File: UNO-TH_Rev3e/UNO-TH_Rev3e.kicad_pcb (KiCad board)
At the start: 2 copper layers, 68.6 x 53.3 mm, 120 parts, among them T1 FDN340P, U1 NCP1117ST50T3G, U2 LP2985-33DBVR, U3 ATMEGA16U2-MU(R), U5 LMV358IDGKR, X1 POWERSUPPLY_DC21MMX, X2 USB-B_TH, Y1 16MHz, Y2 CSTCE16M0V53-R0 16MHZ

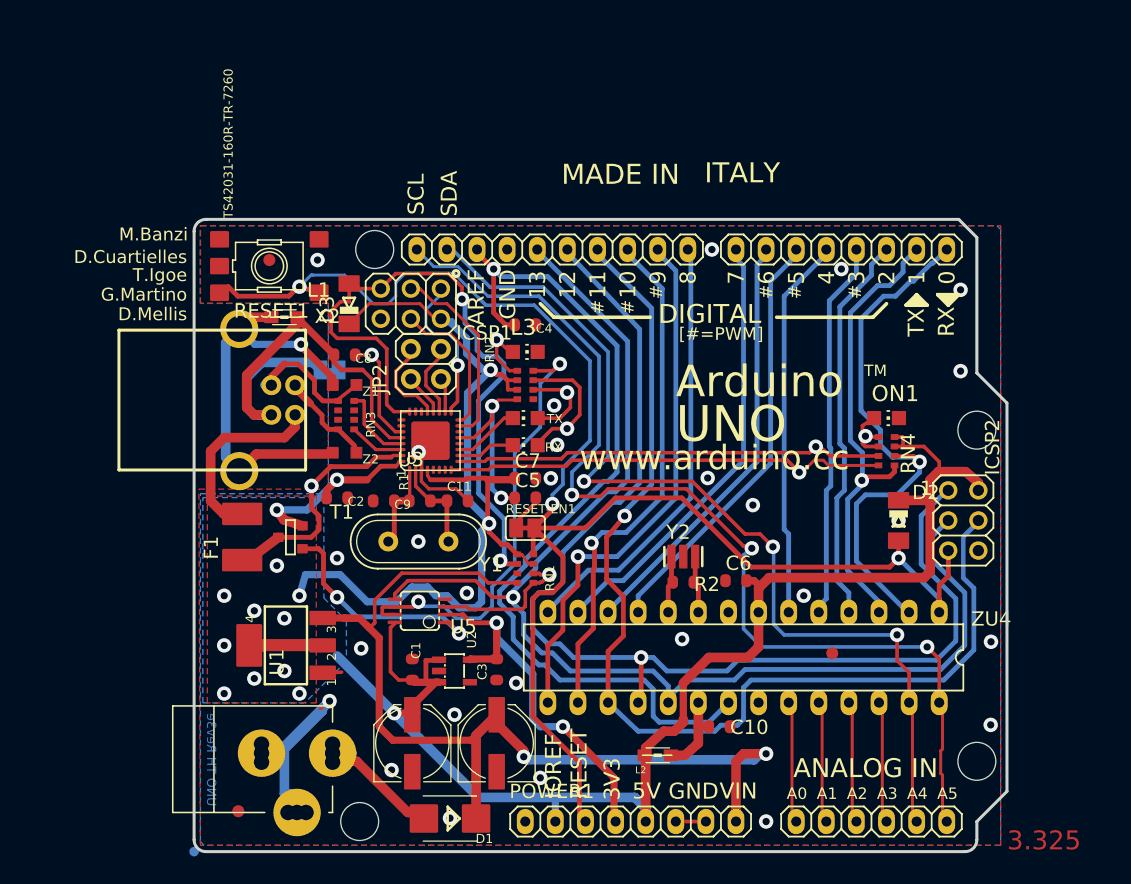
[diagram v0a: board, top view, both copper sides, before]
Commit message: rasp
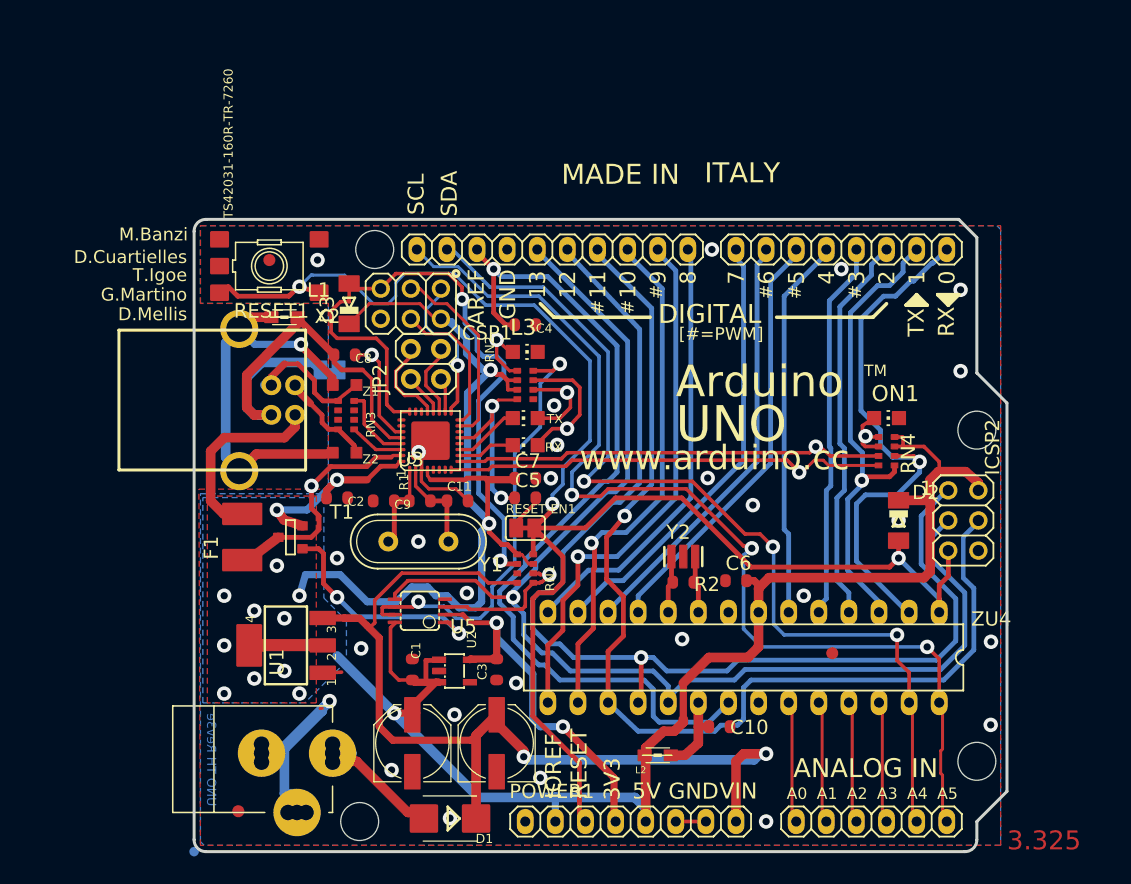
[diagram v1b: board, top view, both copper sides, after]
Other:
- net class Default removed
